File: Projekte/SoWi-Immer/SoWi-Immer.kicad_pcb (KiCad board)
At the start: 2 copper layers, 50 x 16 mm, 17 parts, among them P1 CONN_01X04, U1 SPV1040

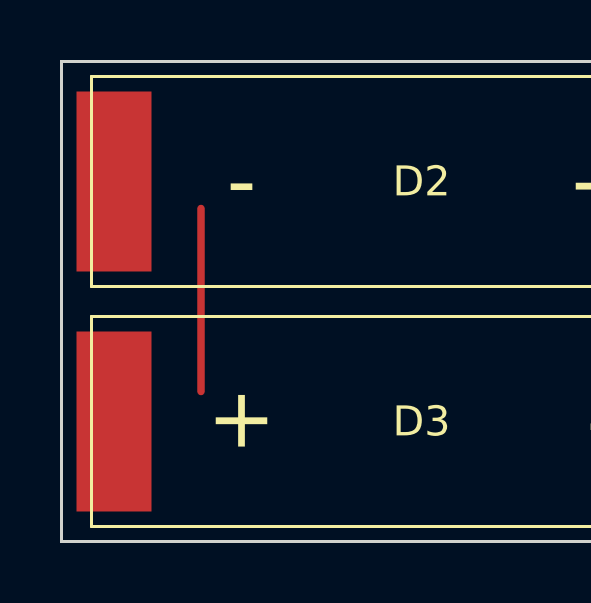
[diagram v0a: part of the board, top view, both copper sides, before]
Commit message: Kléine Laxoutanpassung
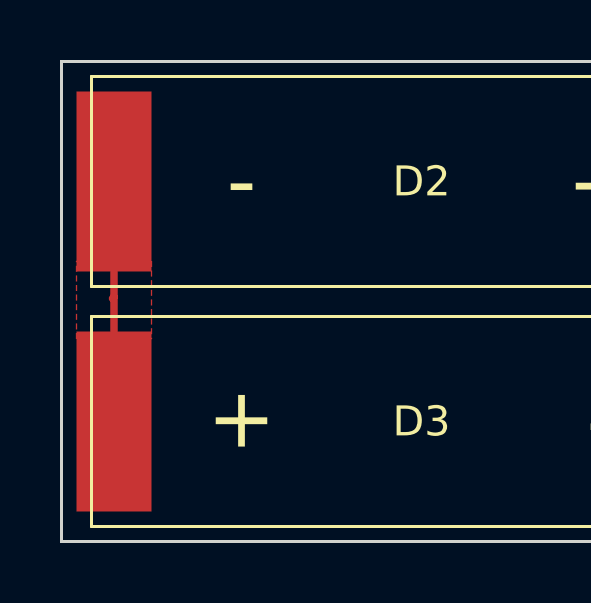
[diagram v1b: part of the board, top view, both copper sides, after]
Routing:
- net Net-(D2-Pad2): track 0.00 -> 8.07 mm
- net (no net): track 6.10 -> 0.00 mm
- added copper zone on F.Cu, net Net-(D2-Pad2)
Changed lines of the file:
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@@
   (general
     (links 30)
-    (no_connects 29)
+    (no_connects 28)
     (area 139.949999 77.949999 190.050001 94.050001)
     (thickness 1.6)
     (drawings 4)
-    (tracks 3)
+    (tracks 5)
     (zones 0)
     (modules 17)
@@
     (last_trace_width 0.25)
     (trace_clearance 0.2)
-    (zone_clearance 0.508)
+    (zone_clearance 0.2)
     (zone_45_only no)
     (trace_min 0.2)
@@
   (gr_line (start 190 78) (end 140 78) (angle 90) (layer Edge.Cuts) (width 0.1))
   (gr_line (start 140 78) (end 140 94) (angle 90) (layer Edge.Cuts) (width 0.1))
-  (segment (start 144.65 82.9) (end 144.65 89) (width 0.25) (layer F.Cu) (net 0))
+  (segment (start 141.75 90) (end 141.75 85.85) (width 0.25) (layer F.Cu) (net 5) (status 400000))
+  (segment (start 141.75 82) (end 141.75 85.85) (width 0.25) (layer F.Cu) (net 5) (status 400000))
+  (segment (start 141.75 85.85) (end 141.7 85.9) (width 0.25) (layer F.Cu) (net 5))
   (segment (start 165.5081 89.008) (end 162.658 89.008) (width 0.25) (layer F.Cu) (net 6))
   (segment (start 162.658 89.008) (end 162.65 89) (width 0.25) (layer F.Cu) (net 6))
+  (zone (net 5) (net_name "Net-(D2-Pad2)") (layer F.Cu) (hatch edge 0.508)
+    (connect_pads yes (clearance 0.2))
+    (min_thickness 0.1)
+    (fill yes (arc_segments 16) (thermal_gap 0.508) (thermal_bridge_width 0.508))
+    (polygon
+      (pts
+        (xy 143 87.25) (xy 140.5 87.25) (xy 140.5 84.65) (xy 143 84.65)
+      )
+    )
+  )
 )
